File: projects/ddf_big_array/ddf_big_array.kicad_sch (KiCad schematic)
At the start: 55 parts, among them J1 Conn_Coaxial, J101 Conn_Coaxial, J102 Conn_Coaxial, J2 Conn_Coaxial, J201 Conn_Coaxial, J202 Conn_Coaxial, J3 Conn_Coaxial, J301 Conn_Coaxial, J302 Conn_Coaxial, J4 Conn_Coaxial, J401 Conn_Coaxial, J402 Conn_Coaxial, J5 Conn_Coaxial, J6 RJ45_Shielded, J7 RJ45_Shielded, J8 Conn_01x05_Male

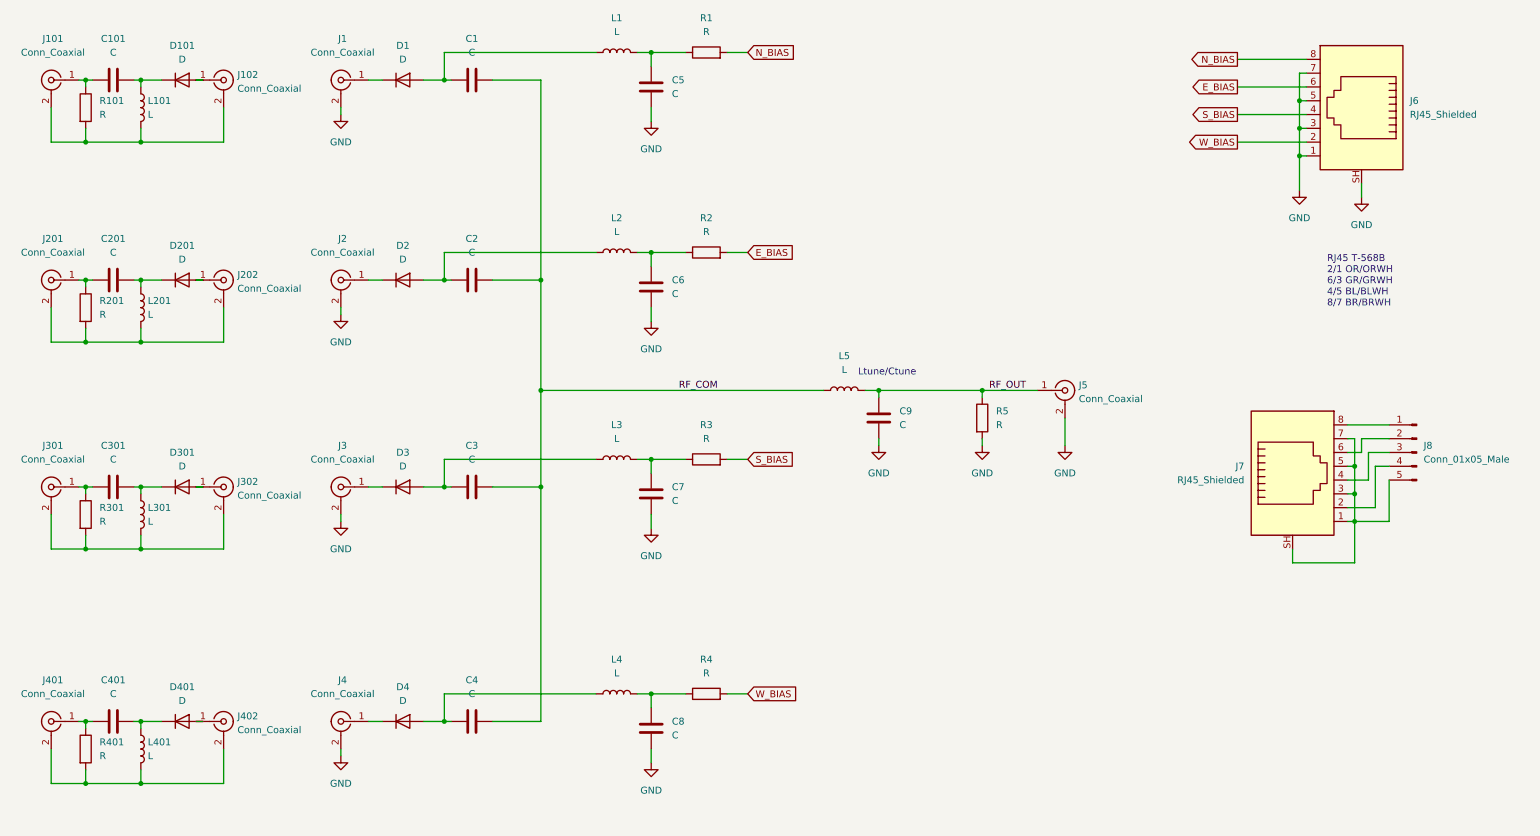
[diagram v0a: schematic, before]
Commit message: Checkpoint.
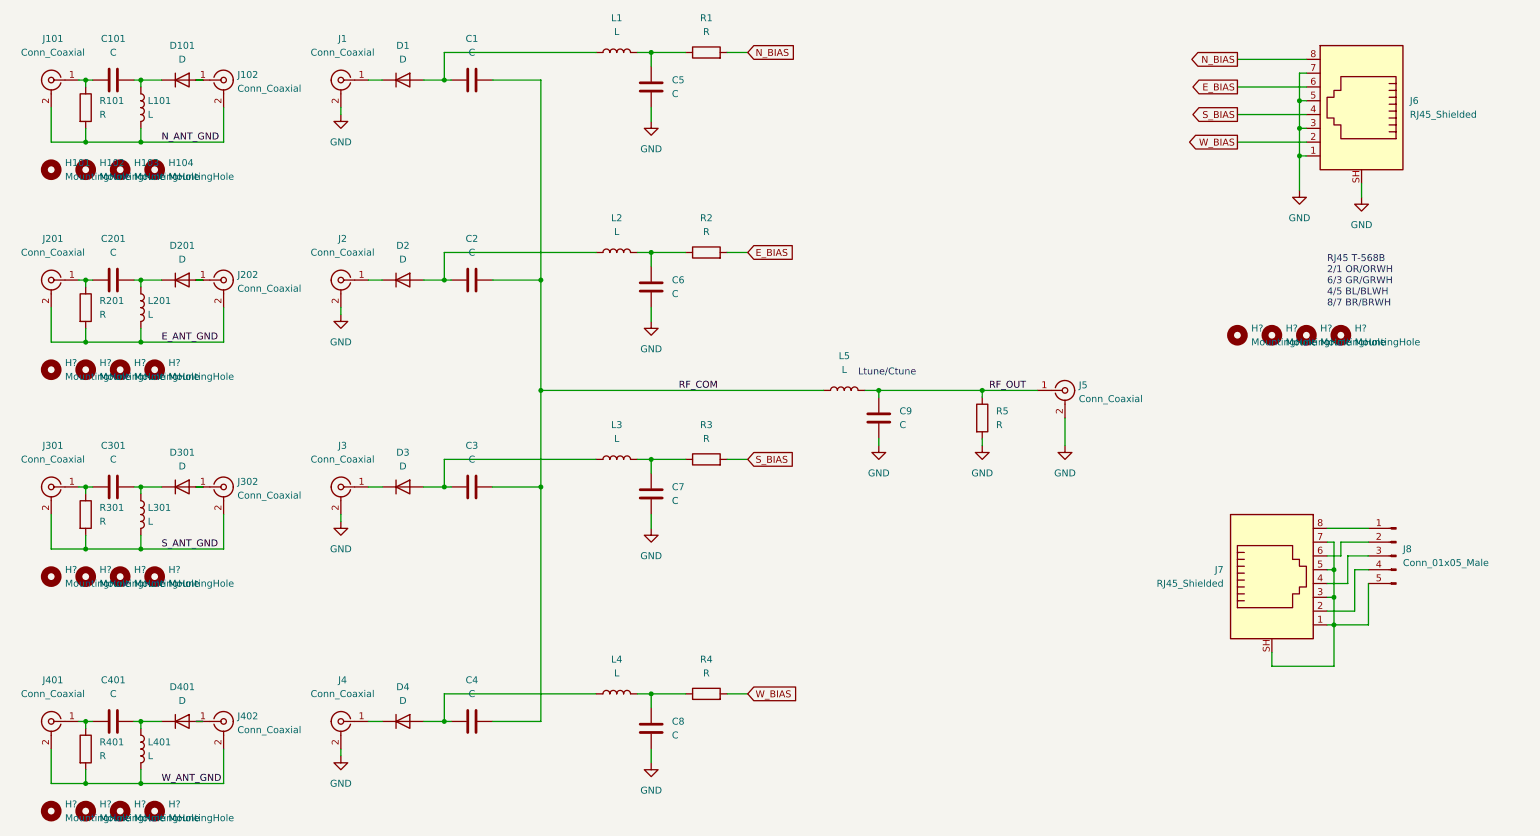
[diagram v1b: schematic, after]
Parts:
- added H101, H102, H103, H104, H? (x16): MountingHole, symbol Mechanical:MountingHole
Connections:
- net W_ANT_GND: now reaches J401.2 (Ext), J402.2 (Ext), L401.2, R401.2
- net E_ANT_GND: now reaches J201.2 (Ext), J202.2 (Ext), L201.2, R201.2
- net S_ANT_GND: now reaches J301.2 (Ext), J302.2 (Ext), L301.2, R301.2
- net N_ANT_GND: now reaches J101.2 (Ext), J102.2 (Ext), L101.2, R101.2
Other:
- moved on the sheet: J7, J8
